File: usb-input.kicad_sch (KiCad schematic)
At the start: 2 parts, among them P1 USB_C_Plug, U1 CH224K

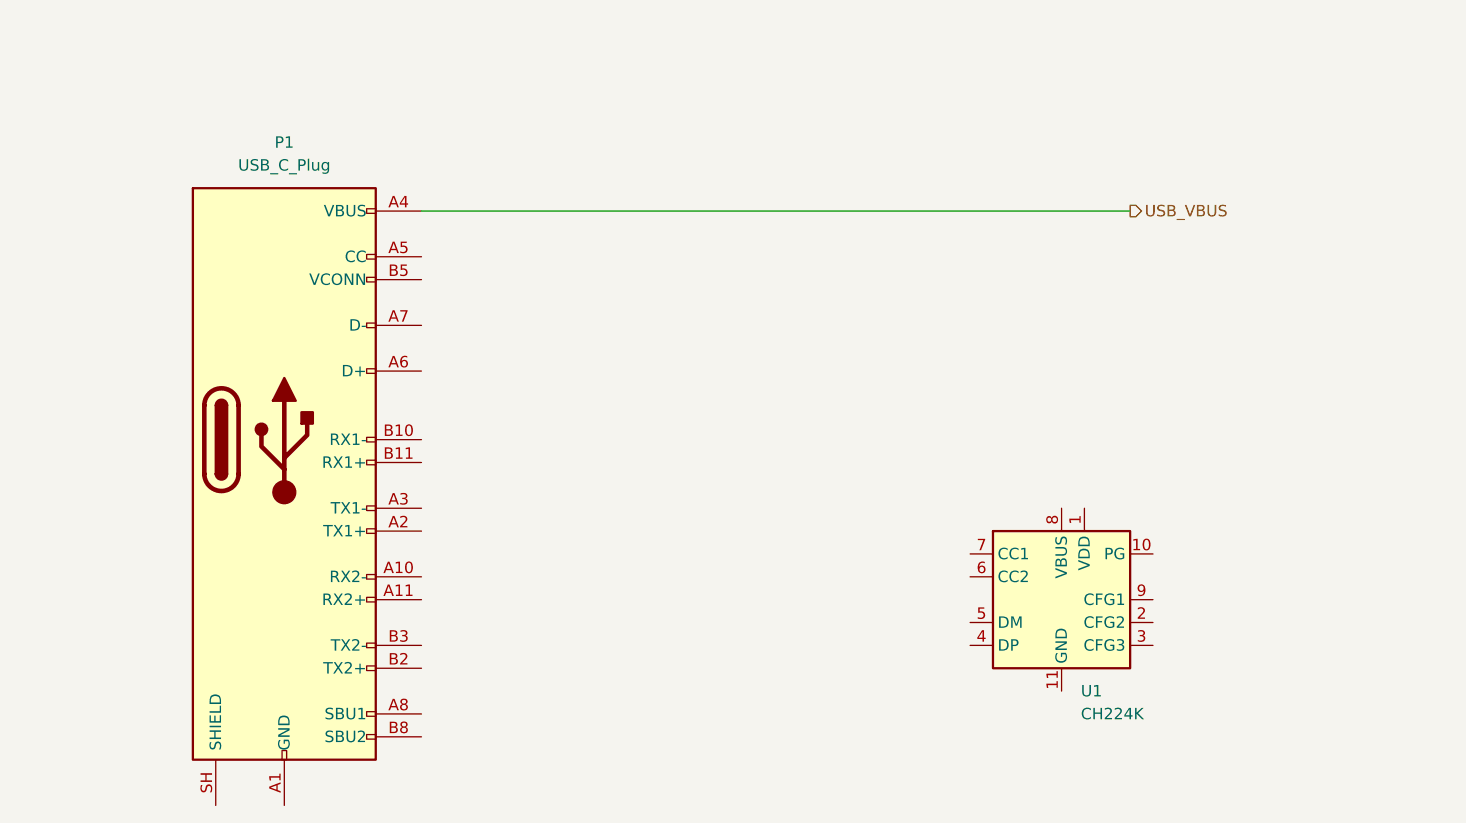
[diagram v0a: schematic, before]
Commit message: uploading
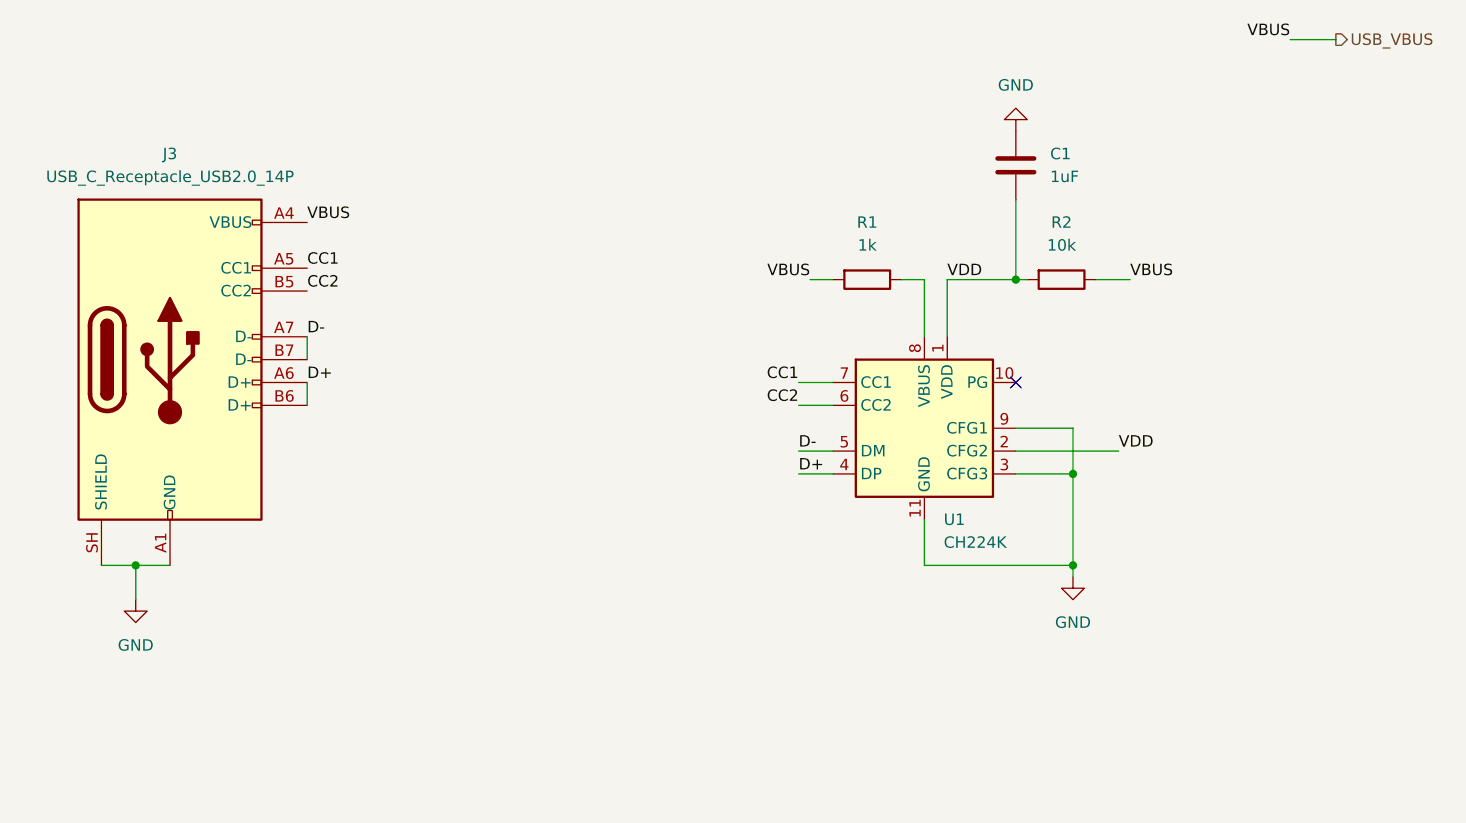
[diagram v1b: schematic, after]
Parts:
- removed P1: USB_C_Plug, symbol Connector:USB_C_Plug
- added C1: 1uF, symbol Device:C
- added J3: USB_C_Receptacle_USB2.0_14P, symbol Connector:USB_C_Receptacle_USB2.0_14P
- added R1: 1k, symbol Device:R
- added R2: 10k, symbol Device:R
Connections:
- net USB_VBUS: now also J3.A4 (VBUS), J3.A9 (VBUS), J3.B4 (VBUS), J3.B9 (VBUS), R1.2, R2.1
- net VDD: now reaches U1.1 (VDD)
- net VDD: now also U1.2 (CFG2), C1.2, R2.2
- net GND: now reaches U1.11 (GND)
- net GND: now also U1.3 (CFG3), U1.9 (CFG1), C1.1, J3.A1 (GND), J3.A12 (GND), J3.B1 (GND), J3.B12 (GND), J3.SH (SHIELD)
- net D+: now reaches U1.4 (DP)
- net D+: now also J3.A6 (D+), J3.B6 (D+)
- net D-: now reaches U1.5 (DM)
- net D-: now also J3.A7 (D-), J3.B7 (D-)
- net CC2: now reaches U1.6 (CC2)
- net CC2: now also J3.B5 (CC2)
- net CC1: now reaches U1.7 (CC1)
- net CC1: now also J3.A5 (CC1)
- net at U1.8 (VBUS): now also R1.1
- no-connect marks 0 -> 1
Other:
- moved on the sheet: U1
